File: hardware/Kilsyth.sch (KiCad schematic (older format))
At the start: 168 parts, among them J1 Conn_JTAG, J10 Conn_02x01, J11 Conn_02x04_Odd_Even, J12 Conn_02x04_Odd_Even, J2 DX07S024JJ2, J3 USB_B_Micro, J4 Conn_02x20_Odd_Even, J5 Conn_02x06_Odd_Even, J6 PUSB3FR4Z, J7 PUSB3FR4Z, J8 Conn_02x06_Odd_Even, J9 Conn_02x06_Odd_Even, SW1 SW_Push, U1 DSC6001CI2A-016.0000T, U2 LFE5U-85F-6BG381C, U3 TPS65261, U5 IS25LP128F-JBLE, U6 FT600Q, U7 AS4C32M16SB, Y1 30MHz ±20ppm

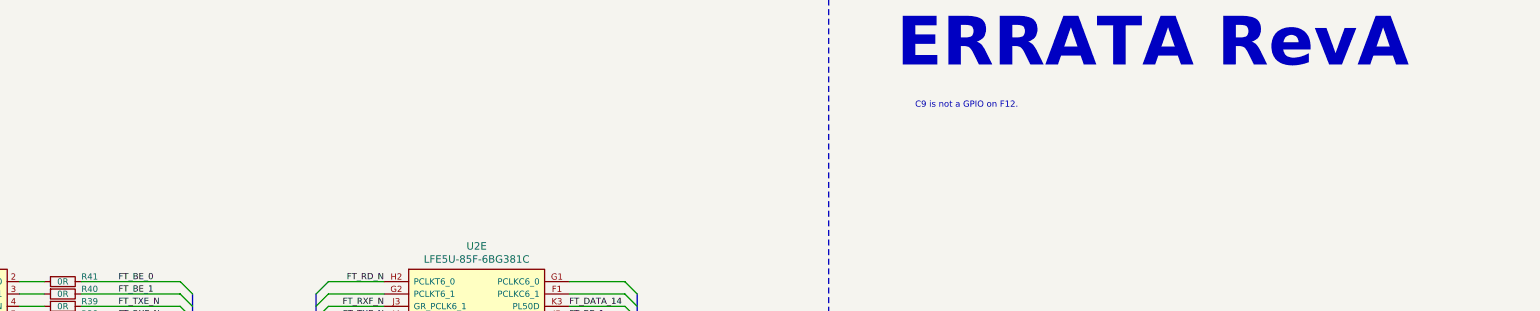
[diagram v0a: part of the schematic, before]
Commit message: Add BODGE information
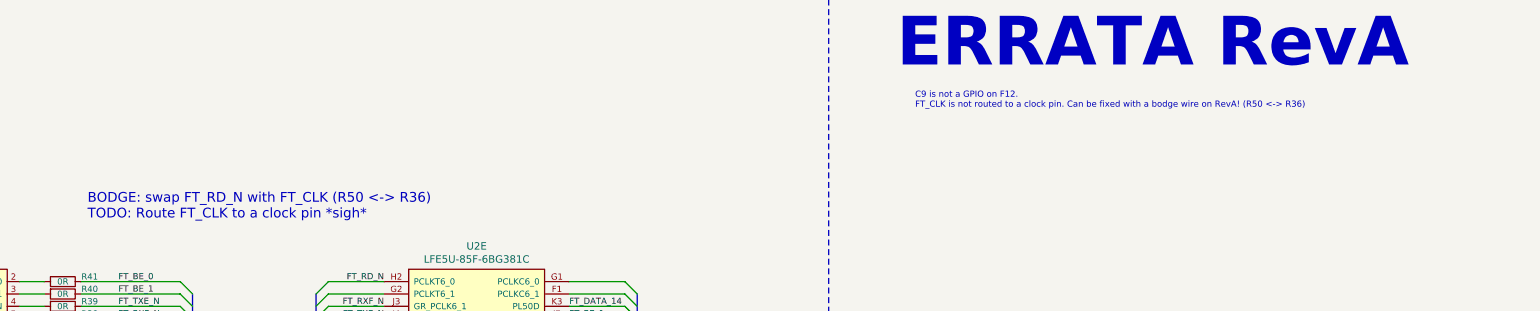
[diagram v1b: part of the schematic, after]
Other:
- note added: "BODGE: swap FT_RD_N with FT_CLK (R50 <-> R36)\nTODO: Route FT_CLK to a clock pin *sigh*"
- note added: "C9 is not a GPIO on F12.\nFT_CLK is not routed to a clock pin. Can be fixed with a bodge wire on RevA! (R50 <-> R36)"
- note removed: "C9 is not a GPIO on F12."
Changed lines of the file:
@@
 ERRATA RevA
 Text Notes 23900 5000 0    50   ~ 0
-C9 is not a GPIO on F12.
+C9 is not a GPIO on F12.\nFT_CLK is not routed to a clock pin. Can be fixed with a bodge wire on RevA! (R50 <-> R36)
 Text Notes 11700 17050 0    50   ~ 0
 FIXME: C9 is not a GPIO on F12.\nRemove pin and move LED to C8
@@
 Wire Bus Line
 	18050 6500 18050 9100
+Text Notes 17200 5900 0    79   ~ 0
+BODGE: swap FT_RD_N with FT_CLK (R50 <-> R36)\nTODO: Route FT_CLK to a clock pin *sigh*
 $EndSCHEMATC
